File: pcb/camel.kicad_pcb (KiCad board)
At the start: 2 copper layers, 75 x 14 mm, 49 parts, among them J1 Conn_01x04, J2 Conn_01x04, Q1 MMBT4403, Q2 MMBT4403, U1 HX711, U2 HX711, U3 MCP1700T-3302E/TT, Y1 11.0592MHz, Y2 11.0592MHz

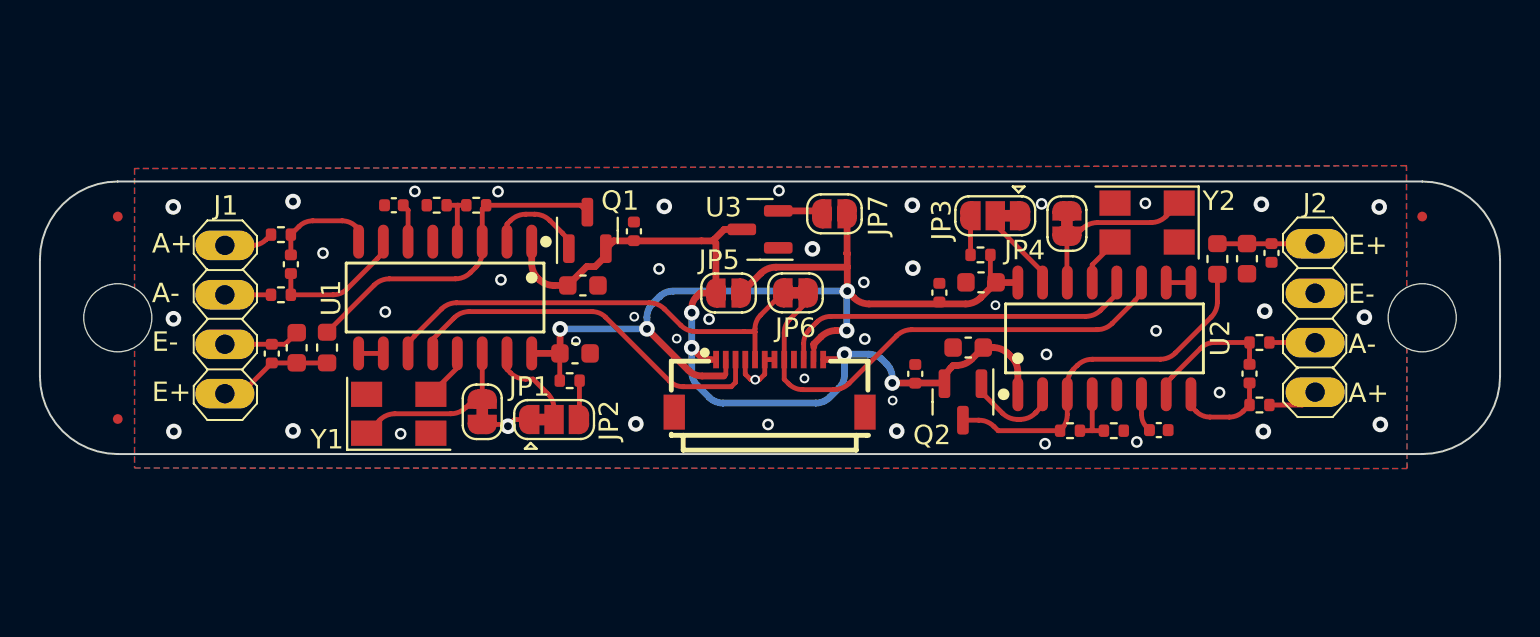
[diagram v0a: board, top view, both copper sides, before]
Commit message: first pass
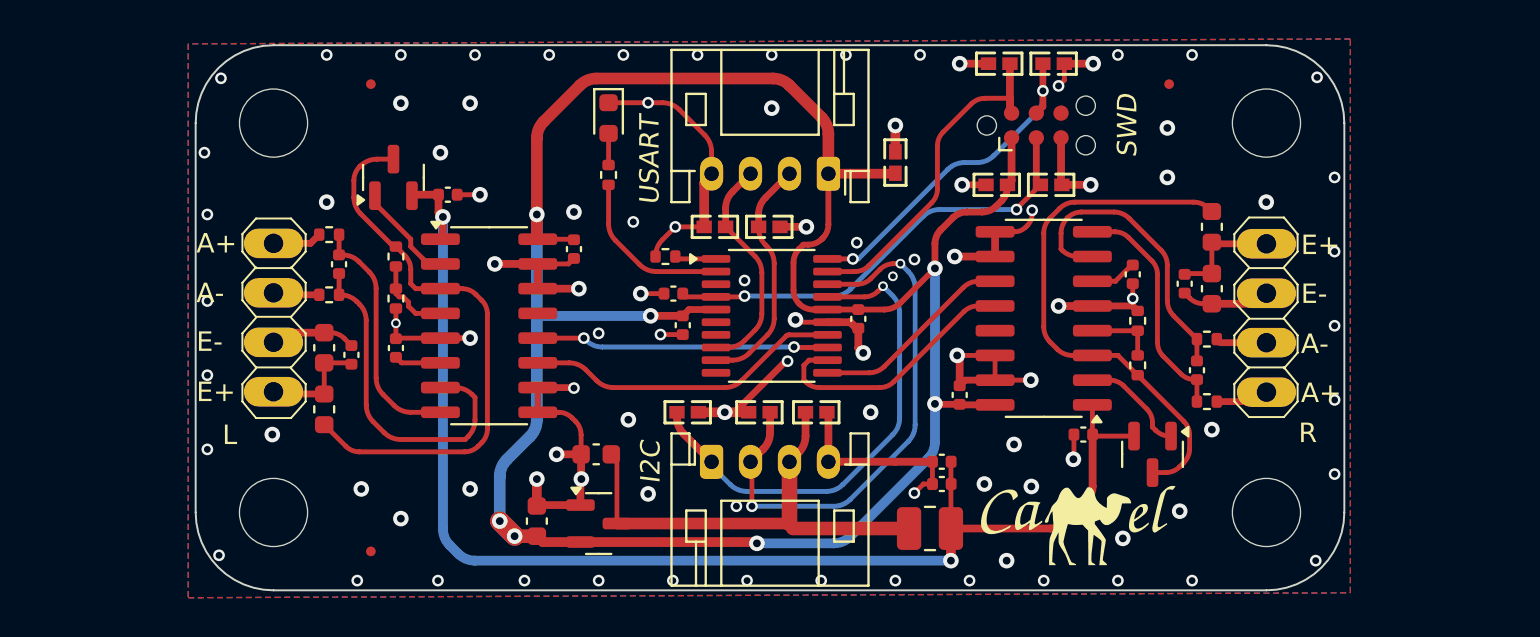
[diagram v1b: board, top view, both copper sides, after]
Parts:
- removed the C13 at (159.3, 103.2)
- removed FPC1: FPC-05F-12PH15, EasyEDA2KiCAD:FPC-SMD_12P-P0.50_XUNPU_FPC-05F-12PH15
- removed JP1, JP4, JP6: SolderJumper_2_Bridged, Jumper:SolderJumper-2_P1.3mm_Bridged_RoundedPad1.0x1.5mm
- removed JP2, JP3: SolderJumper_3_Bridged12, Jumper:SolderJumper-3_P1.3mm_Bridged12_RoundedPad1.0x1.5mm
- removed JP5, JP7: SolderJumper_2_Open, Jumper:SolderJumper-2_P1.3mm_Open_RoundedPad1.0x1.5mm
- removed the R10 at (159.3, 101.8)
- removed the R9 at (138.2, 108.2)
- removed Y1, Y2: 11.0592MHz, Crystal:Crystal_SMD_5032-4Pin_5.0x3.2mm
- added C15: 100n, Capacitor_SMD:C_0402_1005Metric, F.Cu at (143.5, 103.8)
- added C3: 10n, Capacitor_SMD:C_0402_1005Metric, F.Cu at (157.3, 112.4)
- added C4: 1u, Capacitor_SMD:C_0402_1005Metric, F.Cu at (157.3, 113.5)
- added C7: 100n, Capacitor_SMD:C_0402_1005Metric, F.Cu at (138.4, 101.5)
- added C8: 100n, Capacitor_SMD:C_0402_1005Metric, F.Cu at (153.0, 105.1)
- added D1: RED, LED_SMD:LED_0603_1608Metric, F.Cu at (140.2, 94.7)
- added D10: RCLAMP0521P-N, camel:X1-DFN1006-2_L1.0-W0.6-BI, F.Cu at (144.3, 109.9)
- added D11: RCLAMP0521P-N, camel:X1-DFN1006-2_L1.0-W0.6-BI, F.Cu at (148.0, 109.9)
- added D2: RCLAMP0521P-N, camel:X1-DFN1006-2_L1.0-W0.6-BI, F.Cu at (154.9, 97.0)
- added D3: RCLAMP0521P-N, camel:X1-DFN1006-2_L1.0-W0.6-BI, F.Cu at (160.3, 91.9)
- added D4: RCLAMP0521P-N, camel:X1-DFN1006-2_L1.0-W0.6-BI, F.Cu at (163.1, 91.9)
- added D5: RCLAMP0521P-N, camel:X1-DFN1006-2_L1.0-W0.6-BI, F.Cu at (162.9, 98.2)
- added D6: RCLAMP0521P-N, camel:X1-DFN1006-2_L1.0-W0.6-BI, F.Cu at (160.1, 98.2)
- added D7: RCLAMP0521P-N, camel:X1-DFN1006-2_L1.0-W0.6-BI, F.Cu at (148.5, 100.3)
- added D8: RCLAMP0521P-N, camel:X1-DFN1006-2_L1.0-W0.6-BI, F.Cu at (145.7, 100.3)
- added D9: RCLAMP0521P-N, camel:X1-DFN1006-2_L1.0-W0.6-BI, F.Cu at (150.9, 109.9)
- added G***: LOGO, camel:camel_logo_10, F.Cu at (164.3, 115.7)
- added G***: LOGO, camel:camel_logo_10, B.Cu at (147.1, 102.7)
- added H3: MountingHole, MountingHole:MountingHole_3.5mm, F.Cu at (174.0, 95.0)
- added H4: MountingHole, MountingHole:MountingHole_3.5mm, F.Cu at (123.0, 115.0)
- added J2: TC2030-NL, Connector:Tag-Connect_TC2030-IDC-NL_2x03_P1.27mm_Vertical, F.Cu at (162.2, 95.1)
- added J3: USART, Connector_JST:JST_PH_S4B-PH-K_1x04_P2.00mm_Horizontal, F.Cu at (151.5, 97.6)
- added J5: I2C STEMMA, Connector_JST:JST_PH_S4B-PH-K_1x04_P2.00mm_Horizontal, F.Cu at (145.5, 112.4)
- added L1: 39n, Inductor_SMD:L_1008_2520Metric, F.Cu at (156.7, 115.8)
- added R4: 2K2, Resistor_SMD:R_0402_1005Metric, F.Cu at (140.2, 97.7)
- added R8: 10K, Resistor_SMD:R_0402_1005Metric, F.Cu at (143.1, 101.9)
- added U3: STM32L010F4P6, Package_SO:TSSOP-20_4.4x6.5mm_P0.65mm, F.Cu at (148.6, 104.9)
- C10: value 10u -> 100n; footprint Capacitor_SMD:C_0603_1608Metric -> Capacitor_SMD:C_0402_1005Metric
- C9: renamed from C14; value 0.1u -> 100n
- J1: footprint dualScaleBoard_hx711:Pad_1x04_P2.54mm -> camel:Pad_1x04_P2.54mm
- J4: renamed from J2; footprint dualScaleBoard_hx711:Pad_1x04_P2.54mm -> camel:Pad_1x04_P2.54mm
- U2: renamed from U1; footprint EasyEDA2KiCAD:SOP-16_L10.0-W3.9-P1.27-LS6.0-BL -> Package_SO:SOP-16_3.9x9.9mm_P1.27mm
- U4: renamed from U2; footprint EasyEDA2KiCAD:SOP-16_L10.0-W3.9-P1.27-LS6.0-BL -> Package_SO:SOP-16_3.9x9.9mm_P1.27mm
- moved C5 19.9 mm to (139.6, 112.0)
- moved U1 17.2 mm to (139.7, 115.6), turned to 0 degrees
- moved FID1 14.7 mm to (169.0, 93.0)
- moved FID2 14.7 mm to (128.0, 93.0)
- moved FID3 14.7 mm to (128.0, 117.0)
- moved H1 12.8 mm to (123.0, 95.0)
- moved H2 12.8 mm to (174.0, 115.0)
- moved Q1 10.3 mm to (129.2, 97.8)
- moved Q2 10.1 mm to (168.1, 112.0)
- moved C2 9.74 mm to (132.0, 98.7), turned to 0 degrees
- moved C1 9.18 mm to (164.6, 111.0), turned to 180 degrees
- moved C6 8.83 mm to (136.5, 115.4), turned to 90 degrees
- moved C20 8.11 mm to (167.1, 102.8), turned to -90 degrees
- moved C14 7.33 mm to (129.3, 106.6), turned to 90 degrees
- moved R10 5.78 mm to (167.4, 105.2), turned to 90 degrees
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- renumbered C15 to C1, C1 to C11, C3 to C12, C5 to C13, C7 to C14, C2 to C17, C4 to C18, C6 to C19, C9 to C2, C8 to C20, C11 to C5, C12 to C6, H101 to H1, H102 to H2, L1 to L2, L2 to L3, R5 to R1, R8 to R10, R3 to R11, R4 to R12, R6 to R2, R1 to R3, R2 to R5, R7 to R9, U3 to U1
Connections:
- C1 pad 1: VCC -> +5VA
- C10 pad 1: VCC -> +3V3
- C2 pad 1: VCC -> +5VA
- C5 pad 1: VCC -> +5V
- C6 pad 1: VDD -> +3V3
- C9 pad 1: VDD -> +3V3
- Q1 pad 2: VCC -> +5VA
- Q2 pad 2: VCC -> +5VA
- U1 pad 2: /VO -> +3V3
- U1 pad 3: VCC -> +5V
- U2 pad 1: VCC -> +5VA
- U2 pad 13: Net-(U1-XO) -> unconnected-(U2-XO-Pad13)
- U2 pad 14: Net-(JP1-A) -> GND
- U2 pad 15: Net-(JP2-C) -> GND
- U2 pad 16: VDD -> +3V3
- U4 pad 1: VCC -> +5VA
- U4 pad 13: Net-(U2-XO) -> unconnected-(U4-XO-Pad13)
- U4 pad 14: Net-(JP4-A) -> GND
- U4 pad 15: Net-(JP3-C) -> GND
- U4 pad 16: VDD -> +3V3
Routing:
- net +3V3: track 0.00 -> 120.2 mm, vias 0 -> 7
- net GND: track 12.3 -> 109.3 mm, vias 44 -> 99
- net +5VA: track 0.00 -> 66.5 mm, vias 0 -> 2
- net VDD: track 51.7 -> 0.00 mm, vias 4 -> 0
- net VCC: track 47.4 -> 0.00 mm, vias 4 -> 0
- net /I2C_SDA: track 0.00 -> 28.1 mm, vias 0 -> 2
- net /I2C_SCL: track 0.00 -> 25.4 mm, vias 0 -> 1
- net +5V: track 0.00 -> 24.8 mm
- net /NRST: track 0.00 -> 23.2 mm, vias 0 -> 2
- net /SWDIO: track 0.00 -> 18.1 mm
- net /SWCLK: track 0.00 -> 17.6 mm, vias 0 -> 2
- net /SCK2: track 25.8 -> 10.4 mm
- net /USART_TX: track 0.00 -> 12.3 mm
- net /USART_RX: track 0.00 -> 12.3 mm
- net Net-(Q1-C): track 17.6 -> 29.3 mm
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- added copper zone on In1.Cu, net GND
- added copper zone on In2.Cu, net GND
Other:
- board size 75 x 14 mm -> 59 x 28 mm
- copper layers 2 -> 4
- board text added: "3V3"
- board text added: "5V"
- board text added: "GND"
- board text added: "I2C"
- board text added: "L"
- board text added: "R"
- board text added: "RX"
- board text added: "Rev 1.0"
- board text added: "SCL"
- board text added: "SDA"
- board text added: "SWD"
- board text added: "TX"
- board text added: "USART"
- board text removed: "DSBHX711 Rev 1.0"
